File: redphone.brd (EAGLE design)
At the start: 145 x 65 mm, 272 parts, among them IC1 EP4CE6E22, IC10 MPU9250, IC11 PCA9633TK, IC12 HDC1000, IC13 TPS63000, IC14 24LC256, IC16 EPCS4SI8N, IC18 WM8903, IC19 AT25SF041, IC2 STM32F429ZIT, IC20 MP34DT01, IC21 PT4181, IC22 MAX8903A, IC23 NRF24L01, IC24 BME280, IC25 APDS-9960, IC26 DS18B20U, IC27 MC-1010-G, IC28 MAX2659, IC3 MT48LC16M16A2TG, IC4 MAX8815A, IC5 LP3990TL, IC6 LP3990TL, IC7 TPS63001, IC8 ESP8266, IC9 SIM800C, Q1 IRLML2502, Q2 NTA4153NT1G, Q3 BCR133W, Q4 NTA4153NT1G, Q5 NTA4153NT1G, Q6 IRLML2502, Q7 16MHz, Q8 NTA4153NT1G, SW1 PWR, SW2 CAM, SW3 VOL+, SW4 VOL-, X1 MICRO_SIM_SDS, X10 AUDIO-JACKSMD, X13 OV2640, X14 UFL, X16 USB, X18 FPC_I9500_BAT_CON, X3 RM68120_LCD, X5 LG_P715_TS, Y1 2.4Ghz, Y3 2.4Ghz, Y4 GSM_PCB, Y5 2.4Ghz

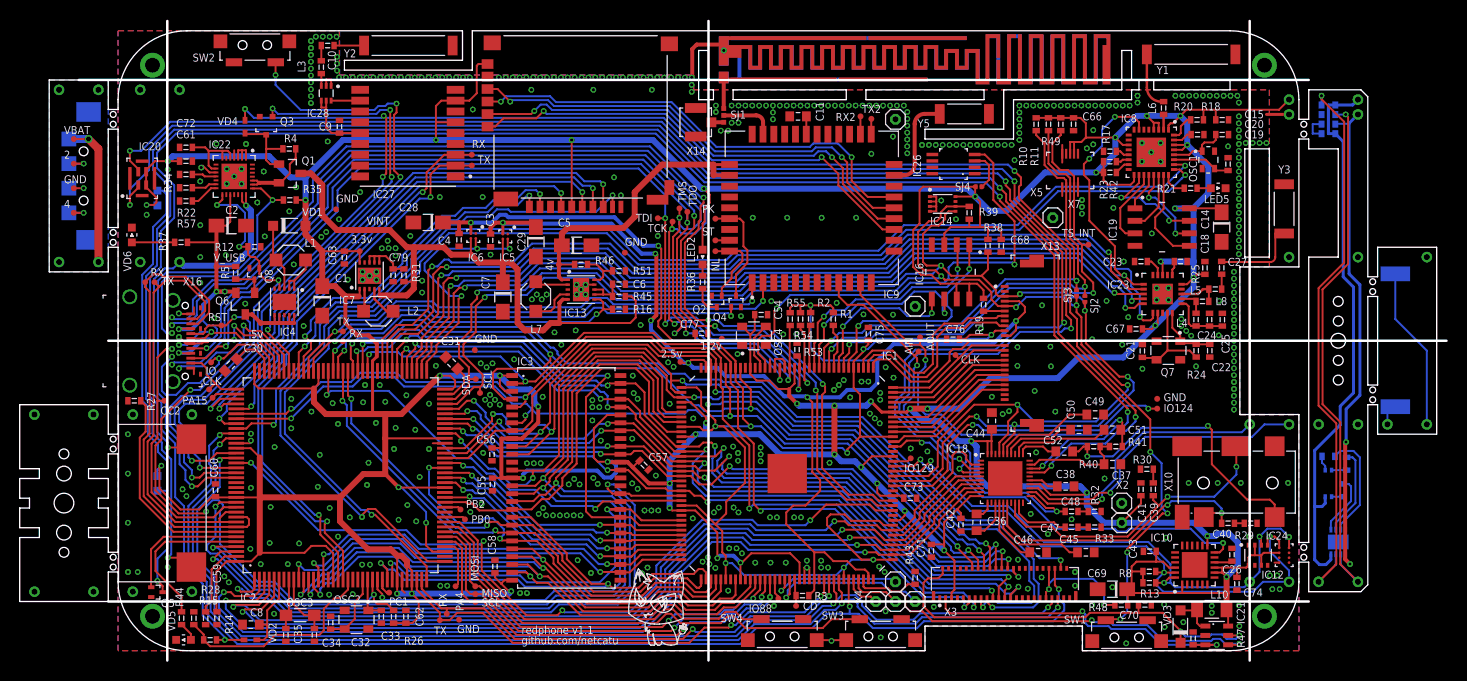
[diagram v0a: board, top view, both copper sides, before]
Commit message: fix MPU9250 pkg
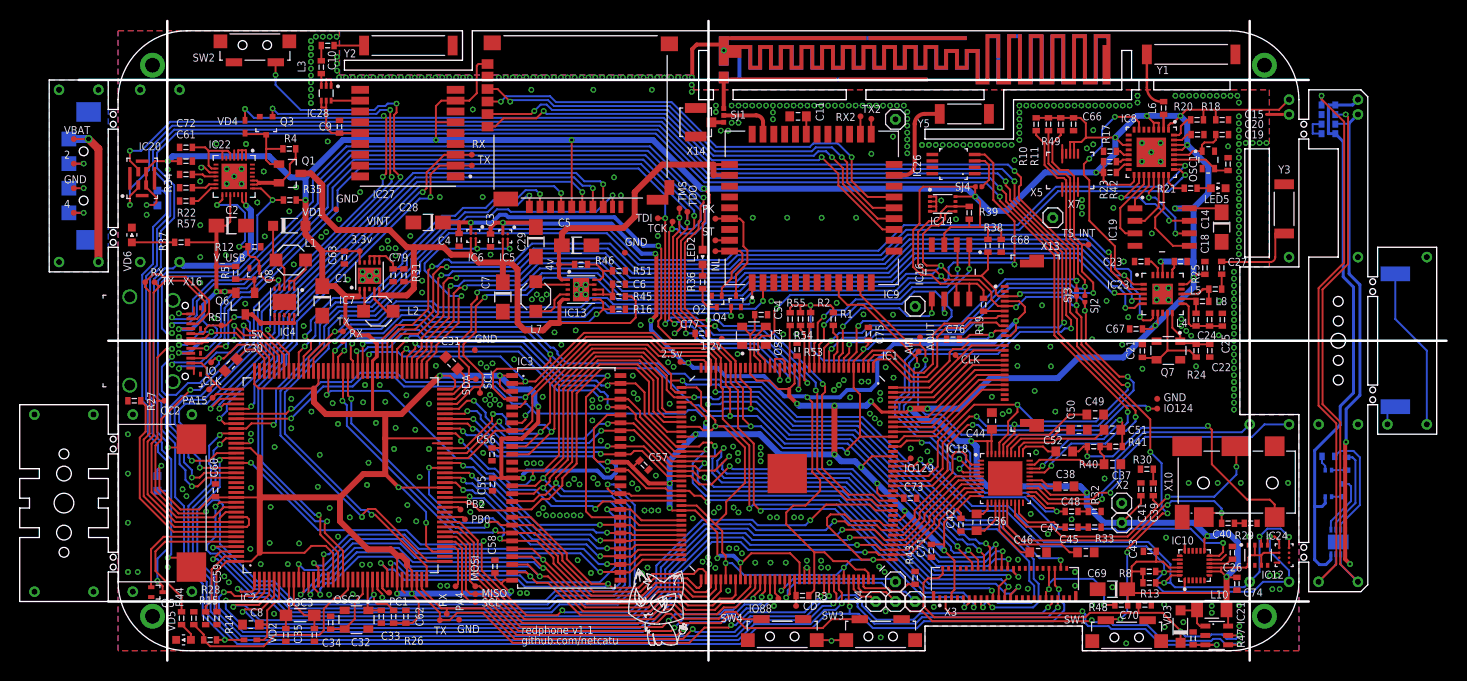
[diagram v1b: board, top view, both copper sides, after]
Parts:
- IC10: device netcat:QFN24-EP -> netcat:QFN24-3X3
- SJ1: value SJ3 -> (none)
- moved C26 0.21 mm to (113.2, 9.95)
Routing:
- net GND: track 45.0 -> 48.2 mm
- net 3.3V: track 792.5 -> 795.0 mm
- net NAV_INT0: track 40.3 -> 41.1 mm
- net N$78: track 1.83 -> 2.54 mm
- net NAV_I2C_SDA: track 57.3 -> 57.8 mm
- net NAV_I2C_SCL: track 59.1 -> 59.6 mm
